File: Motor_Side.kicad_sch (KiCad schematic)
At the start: 32 parts, among them U2 TLV9301xDCK, U3 TLV9301xDCK, U4 TCMT1106, U5 TCMT1106

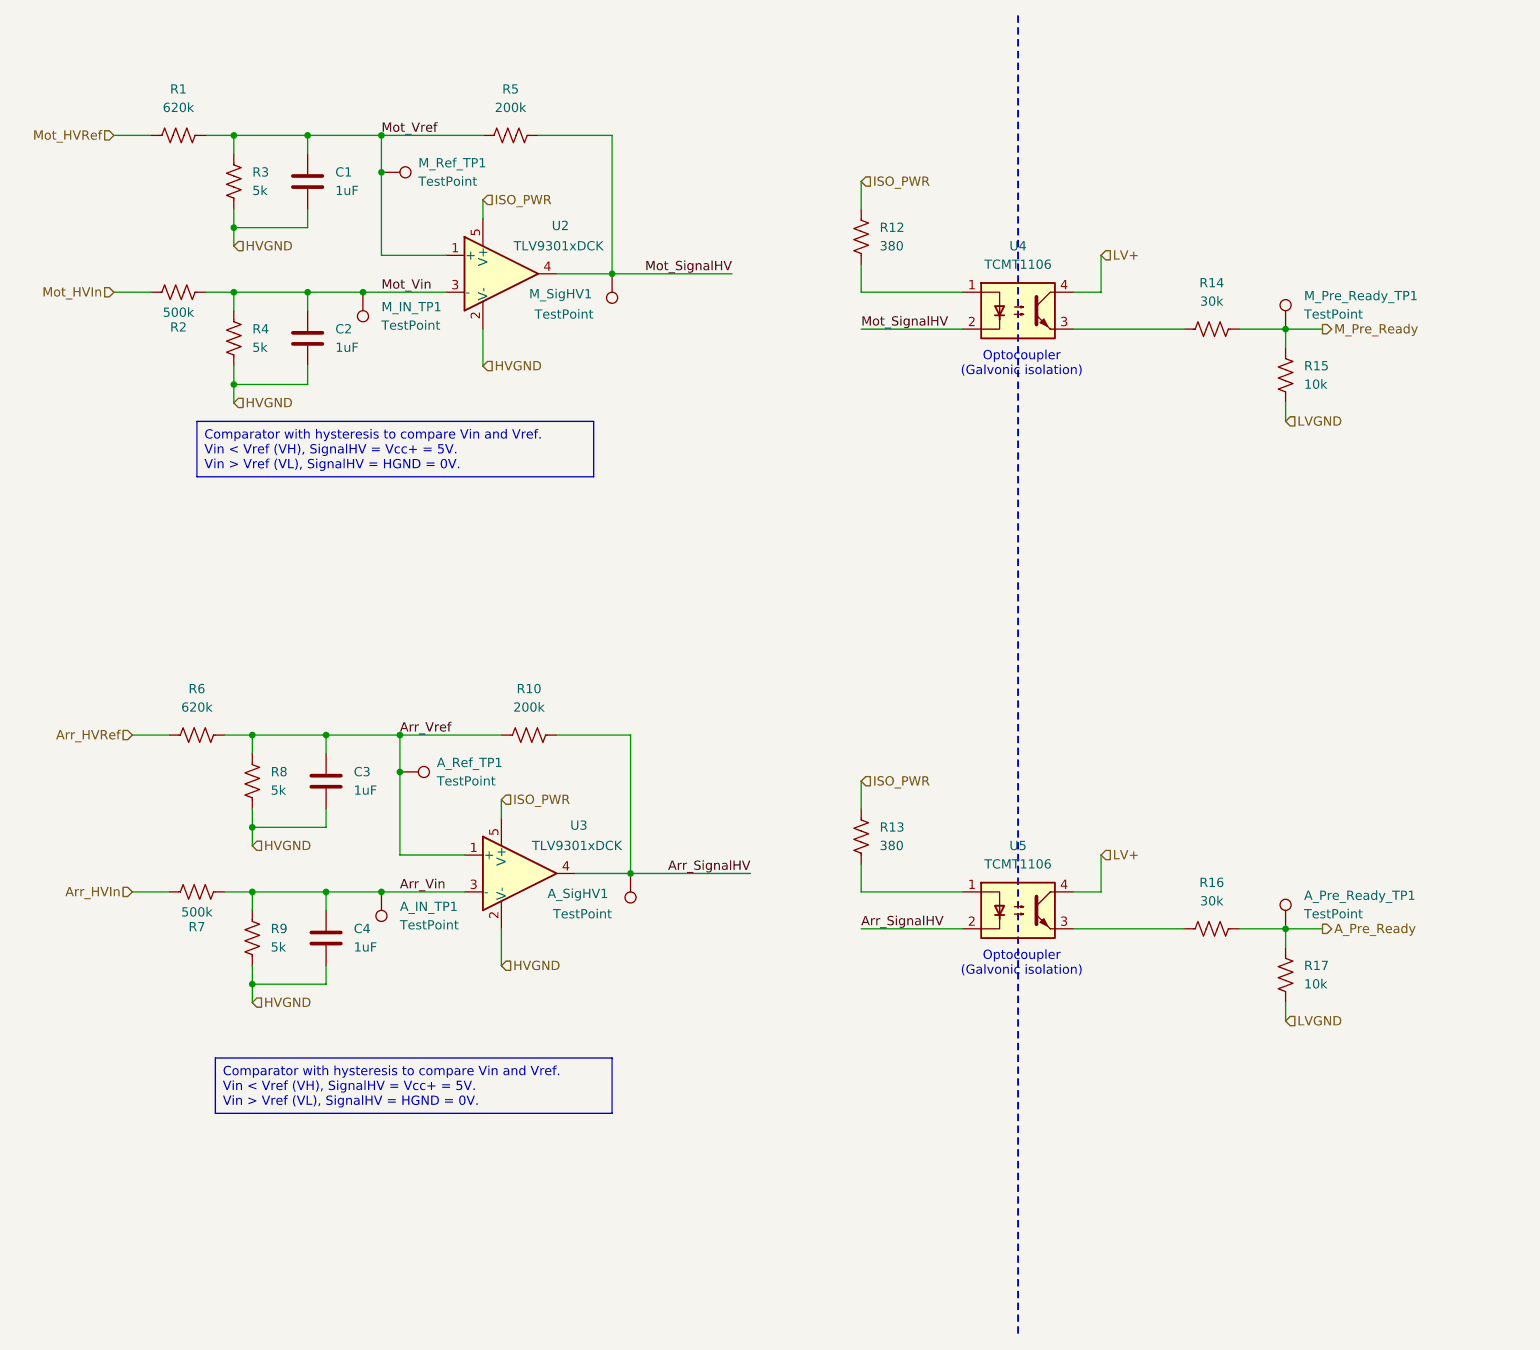
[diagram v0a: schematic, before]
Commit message: initial commit v2
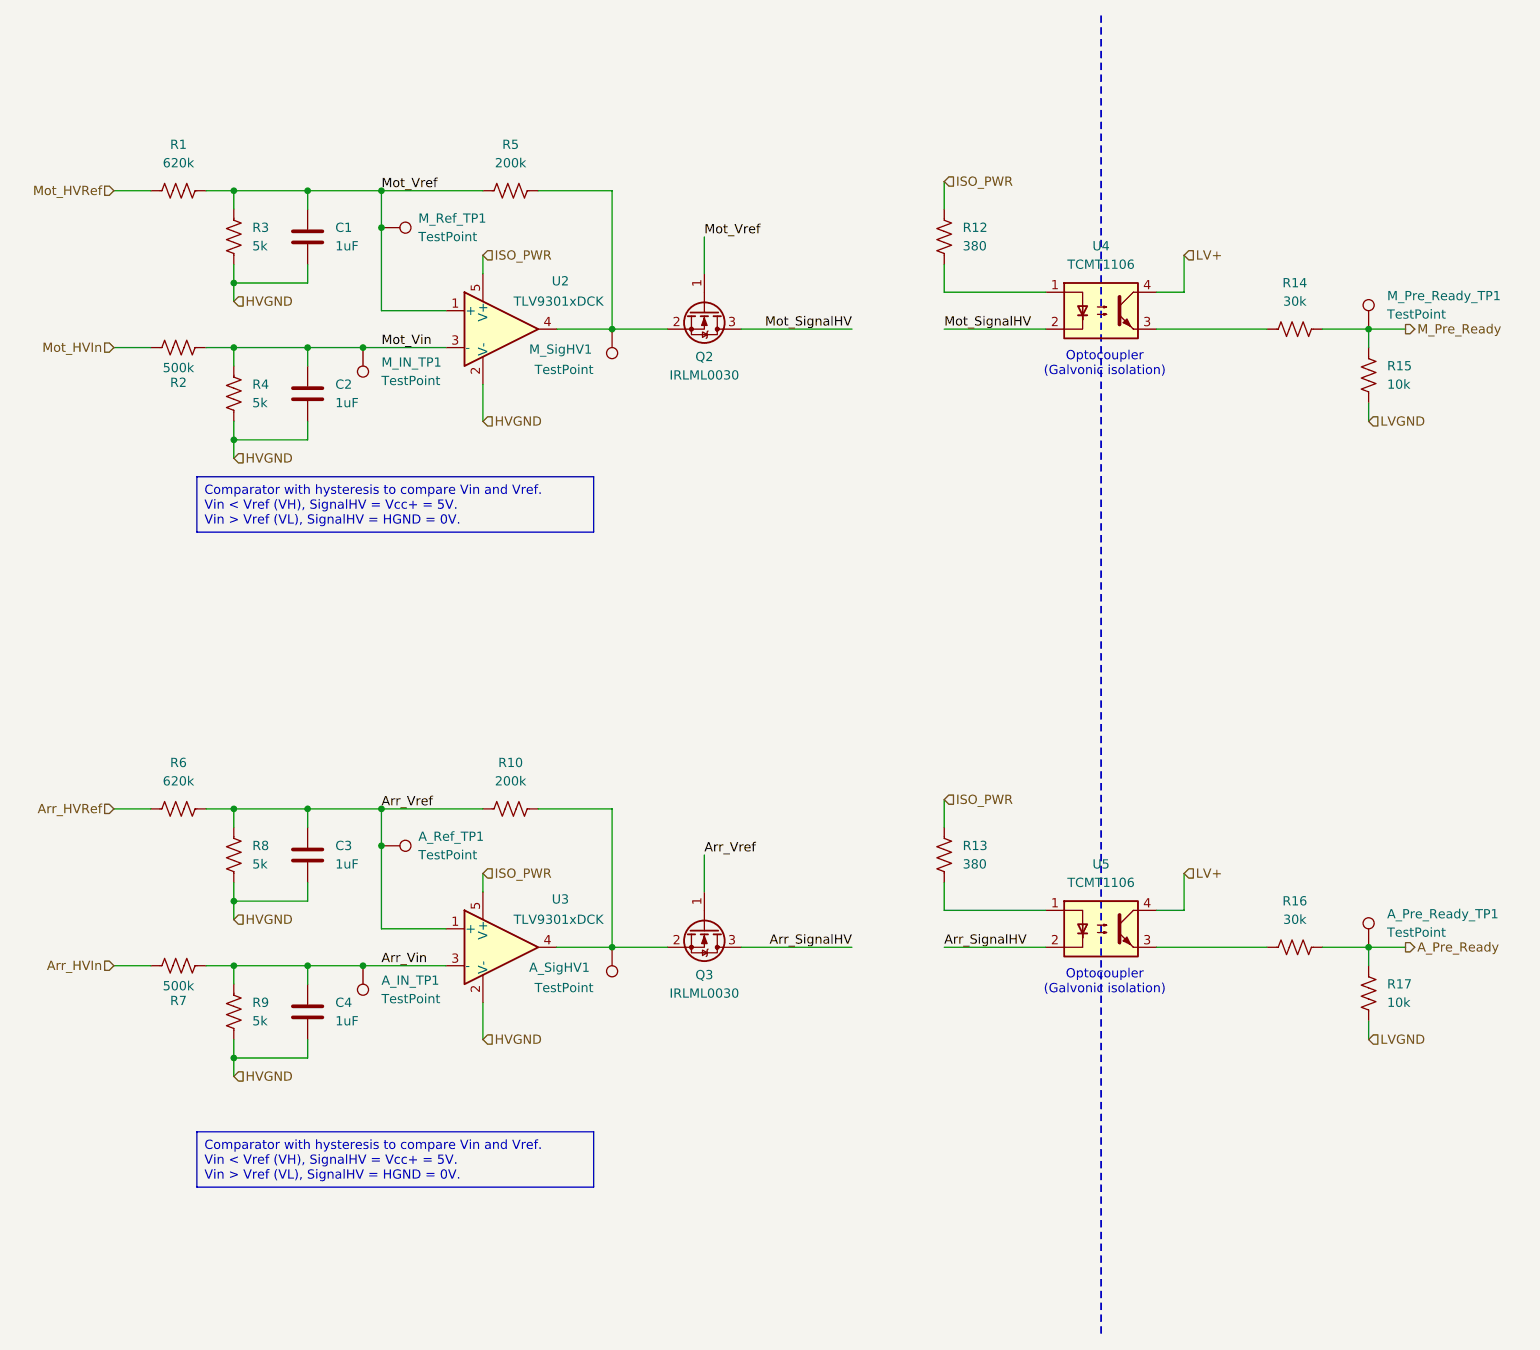
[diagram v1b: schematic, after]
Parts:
- added Q2, Q3: IRLML0030, Package_TO_SOT_SMD:SOT-23, symbol Transistor_FET:IRLML0030
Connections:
- net Arr_SignalHV: now also Q3.3 (D); no longer A_SigHV1.1, R10.1, U3.4
- net Arr_Vref: now also Q3.1 (G)
- net Mot_SignalHV: now also Q2.3 (D); no longer M_SigHV1.1, R5.1, U2.4
- net Mot_Vref: now also Q2.1 (G)
- new net: A_SigHV1.1, Q3.2 (S), R10.1, U3.4
- new net: M_SigHV1.1, Q2.2 (S), R5.1, U2.4
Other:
- moved on the sheet: A_IN_TP1, A_Pre_Ready_TP1, A_Ref_TP1, A_SigHV1, C1, C2, C3, C4, M_IN_TP1, M_Pre_Ready_TP1, M_Ref_TP1, M_SigHV1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
